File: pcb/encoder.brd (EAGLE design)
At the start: 80 x 36 mm, 41 parts, among them SW1 EC12E_SW, SW2 EC12E_SW, SW3 EC12E_SW, SW4 EC12E_SW, X1 IGRID-14

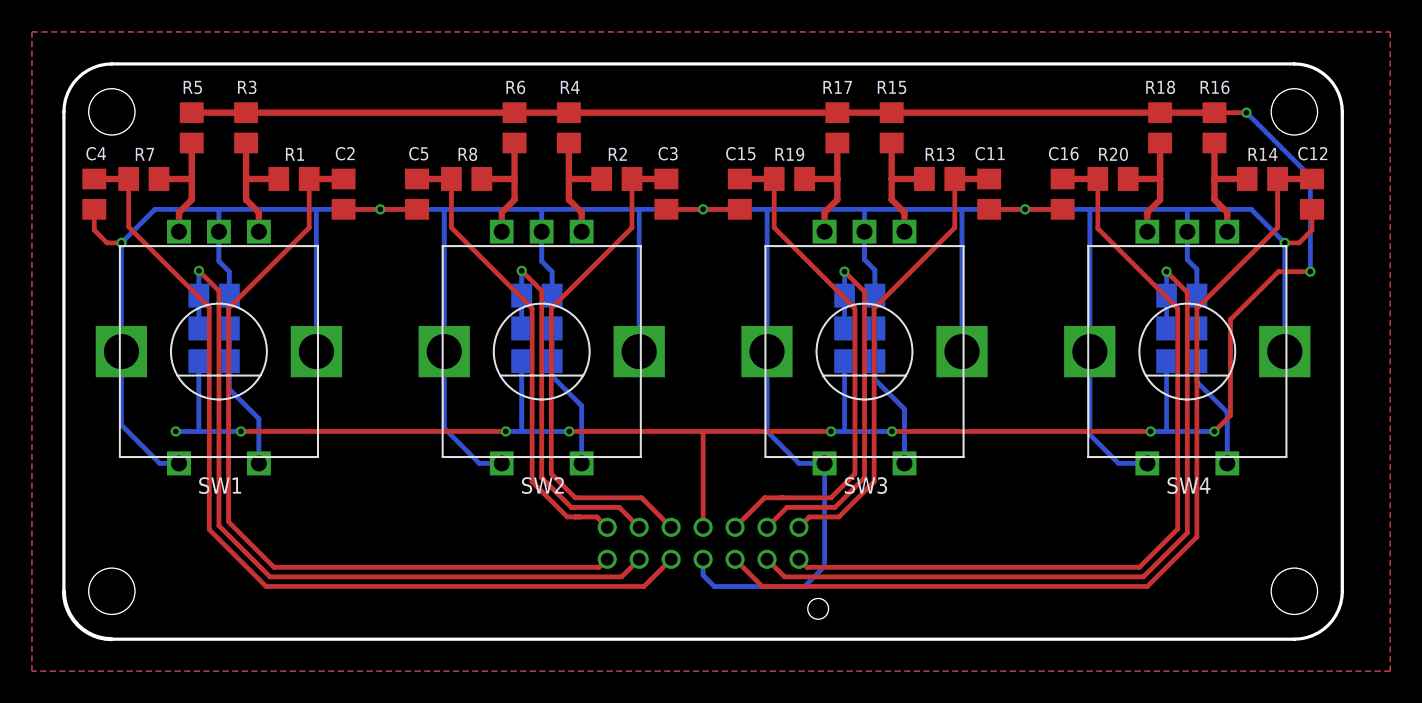
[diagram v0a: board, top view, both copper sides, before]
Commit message: iron drills deleted
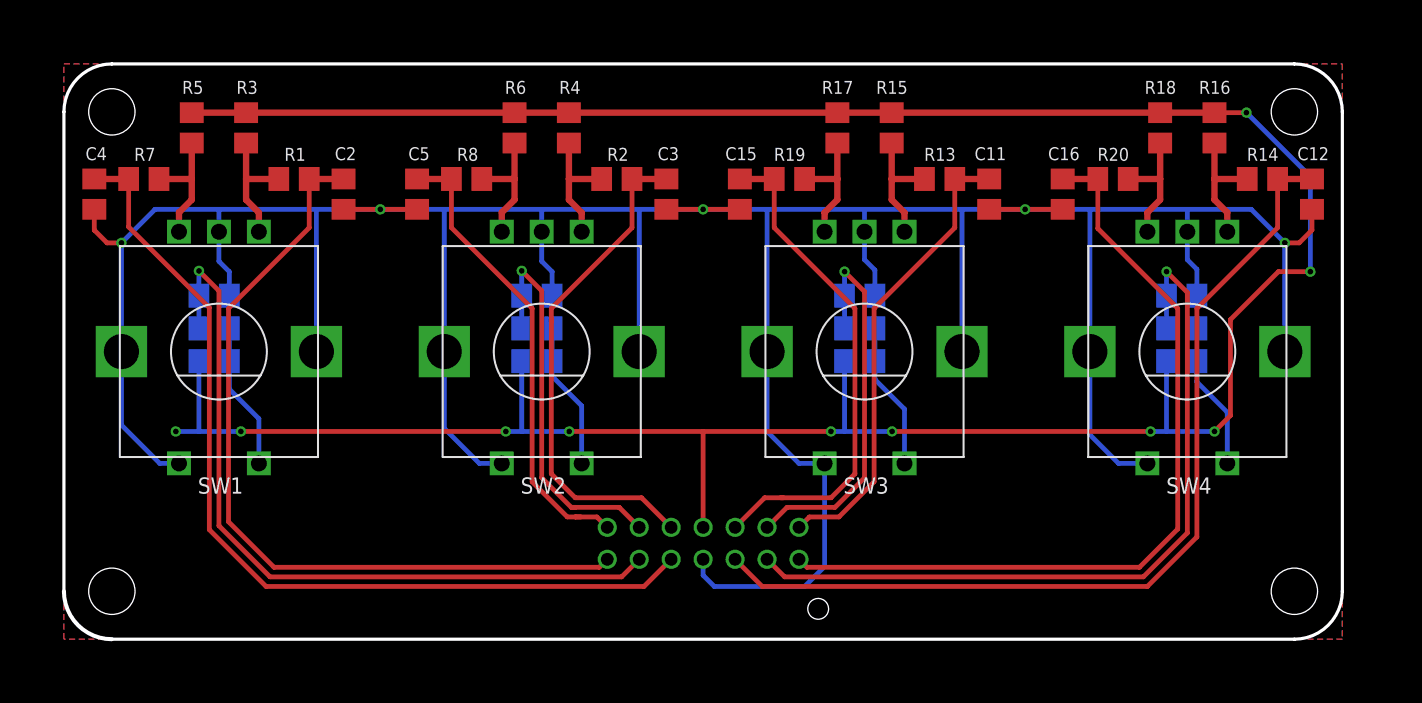
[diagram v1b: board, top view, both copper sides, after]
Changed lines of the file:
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@@
 <?xml version="1.0" encoding="utf-8"?>
 <!DOCTYPE eagle SYSTEM "eagle.dtd">
-<eagle version="9.0.1">
+<eagle version="9.3.0">
 <drawing>
 <settings>
@@
 <param name="checkStop" value="0"/>
 <param name="checkValues" value="0"/>
+<param name="checkNames" value="1"/>
+<param name="checkWireStubs" value="1"/>
+<param name="checkPolygonWidth" value="0"/>
 <param name="useDiameter" value="13"/>
 <param name="maxErrors" value="50"/>
@@
 <contactref element="C17" pad="2"/>
 <polygon width="0.4" layer="16" isolate="0.3048">
-<vertex x="-2" y="38"/>
-<vertex x="83" y="38"/>
-<vertex x="83" y="-2"/>
-<vertex x="-2" y="-2"/>
+<vertex x="0" y="36"/>
+<vertex x="80" y="36"/>
+<vertex x="80" y="0"/>
+<vertex x="0" y="0"/>
 </polygon>
 <contactref element="SW1" pad="E"/>
@@
 <contactref element="R21" pad="2"/>
 <polygon width="0.4" layer="1" isolate="0.3048">
-<vertex x="-2" y="38"/>
-<vertex x="83" y="38"/>
-<vertex x="83" y="-2"/>
-<vertex x="-2" y="-2"/>
+<vertex x="0" y="36"/>
+<vertex x="80" y="36"/>
+<vertex x="80" y="0"/>
+<vertex x="0" y="0"/>
 </polygon>
 <wire x1="8" y1="32.95" x2="11.4" y2="32.95" width="0.4" layer="1"/>
@@
 </signal>
 </signals>
+<mfgpreviewcolors>
+<mfgpreviewcolor name="soldermaskcolor" color="0xC8008000"/>
+<mfgpreviewcolor name="silkscreencolor" color="0xFFFEFEFE"/>
+<mfgpreviewcolor name="backgroundcolor" color="0xFF282828"/>
+<mfgpreviewcolor name="coppercolor" color="0xFFFFBF00"/>
+<mfgpreviewcolor name="substratecolor" color="0xFF786E46"/>
+</mfgpreviewcolors>
 </board>
 </drawing>
